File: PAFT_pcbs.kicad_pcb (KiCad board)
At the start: 4 copper layers, 65 x 56.5 mm, 41 parts, among them J1 Servo_R, J10 LinearPotR, J2 Servo_L, J3 Conn_02x03_Top_Bottom, J4 Actuator_L, J5 Actuator_R, J6 RPi_GPIO, J7 LinearPotL, J8 12V_In, J9 RPi_Terminal, SW1 SW_Push, U1 LM2596T-ADJ/LF02, U3 ATtiny85-20P, U4 DRV8848PWP

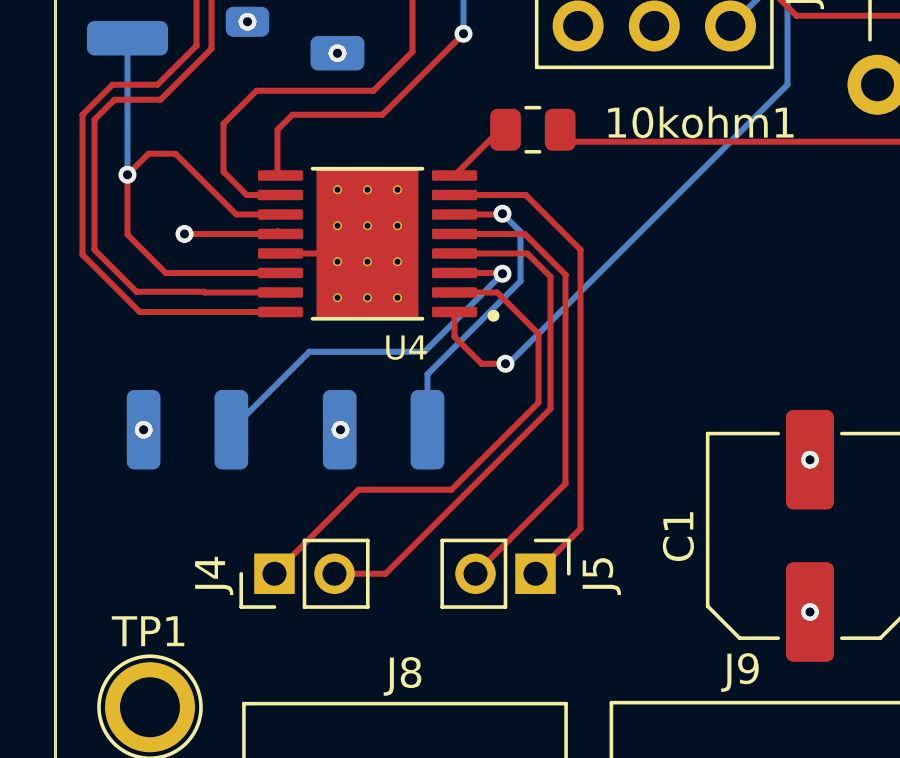
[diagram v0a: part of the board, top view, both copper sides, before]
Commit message: Final updates
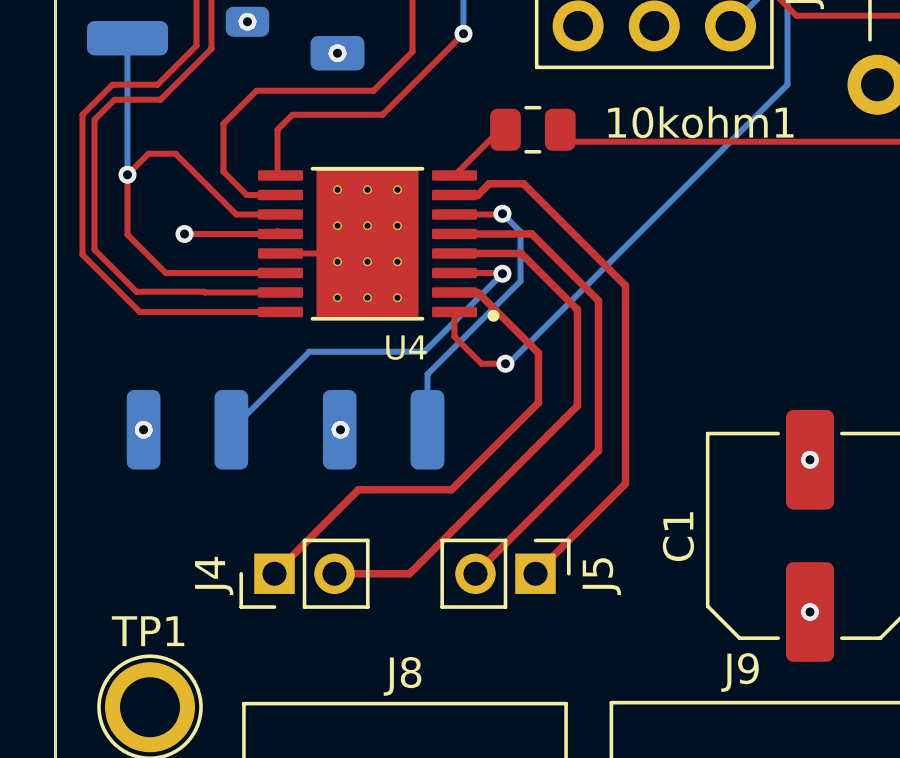
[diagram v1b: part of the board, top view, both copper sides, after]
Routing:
- net /HBridge/BOUT1: track 16.4 -> 18.1 mm
- net /HBridge/AOUT2: track 17.4 -> 18.5 mm
- net /HBridge/BOUT2: track 15.5 -> 16.5 mm
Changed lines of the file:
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@@
 		)
 		(pad_to_mask_clearance 0)
-		(solder_mask_min_width 0.0762)
 		(allow_soldermask_bridges_in_footprints no)
 		(tenting front back)
@@
 			(outputformat 1)
 			(mirror no)
-			(drillshape 1)
+			(drillshape 0)
 			(scaleselection 1)
-			(outputdirectory "")
+			(outputdirectory "../Downloads/")
 		)
 	)
@@
 	)
 	(segment
-		(start 82.3 105)
-		(end 85.2 102.1)
-		(width 0.2)
+		(start 79.2 105)
+		(end 82.3 105)
+		(width 0.25)
 		(layer "F.Cu")
 		(net 18)
 	)
 	(segment
-		(start 85.2 99.8)
-		(end 83.825 98.425)
-		(width 0.2)
+		(start 76.4 107.8)
+		(end 79.2 105)
+		(width 0.25)
 		(layer "F.Cu")
 		(net 18)
 	)
 	(segment
-		(start 83.825 98.425)
-		(end 82.4 98.425)
-		(width 0.2)
+		(start 82.3 105)
+		(end 85.2 102.1)
+		(width 0.25)
 		(layer "F.Cu")
 		(net 18)
 	)
 	(segment
-		(start 85.2 102.1)
-		(end 85.2 99.8)
-		(width 0.2)
+		(start 83.182328 98.425)
+		(end 82.4 98.425)
+		(width 0.25)
 		(layer "F.Cu")
 		(net 18)
 	)
 	(segment
-		(start 79.2 105)
-		(end 82.3 105)
-		(width 0.2)
+		(start 85.2 100.442672)
+		(end 83.182328 98.425)
+		(width 0.25)
 		(layer "F.Cu")
 		(net 18)
 	)
 	(segment
-		(start 76.4 107.8)
-		(end 79.2 105)
-		(width 0.2)
+		(start 85.2 102.1)
+		(end 85.2 100.442672)
+		(width 0.25)
 		(layer "F.Cu")
 		(net 18)
 	)
 	(segment
-		(start 84.825 97.125)
-		(end 85.6 97.9)
-		(width 0.2)
+		(start 86.5 99)
+		(end 86.5 102.2)
+		(width 0.25)
 		(layer "F.Cu")
 		(net 19)
 	)
 	(segment
-		(start 80.1 107.8)
+		(start 80.9 107.8)
 		(end 78.4 107.8)
-		(width 0.2)
+		(width 0.25)
 		(layer "F.Cu")
 		(net 19)
 	)
 	(segment
-		(start 85.6 97.9)
-		(end 85.6 102.3)
-		(width 0.2)
+		(start 86.5 102.2)
+		(end 80.9 107.8)
+		(width 0.25)
 		(layer "F.Cu")
 		(net 19)
 	)
 	(segment
-		(start 85.6 102.3)
-		(end 80.1 107.8)
-		(width 0.2)
+		(start 82.4 97.125)
+		(end 84.625 97.125)
+		(width 0.25)
 		(layer "F.Cu")
 		(net 19)
 	)
 	(segment
-		(start 82.4 97.125)
-		(end 84.825 97.125)
-		(width 0.2)
+		(start 84.625 97.125)
+		(end 86.5 99)
+		(width 0.25)
 		(layer "F.Cu")
 		(net 19)
 	)
 	(segment
-		(start 84.775 95.175)
-		(end 82.4 95.175)
-		(width 0.2)
+		(start 82.4 95.175)
+		(end 83.182328 95.175)
+		(width 0.25)
 		(layer "F.Cu")
 		(net 20)
 	)
 	(segment
-		(start 85.1 107.8)
-		(end 86.6 106.3)
-		(width 0.2)
+		(start 83.557328 94.8)
+		(end 84.7 94.8)
+		(width 0.25)
 		(layer "F.Cu")
 		(net 20)
 	)
 	(segment
-		(start 86.6 97)
-		(end 84.775 95.175)
-		(width 0.2)
+		(start 88.1 98.2)
+		(end 88.1 104.8)
+		(width 0.25)
 		(layer "F.Cu")
 		(net 20)
 	)
 	(segment
-		(start 86.6 106.3)
-		(end 86.6 97)
-		(width 0.2)
+		(start 83.182328 95.175)
+		(end 83.557328 94.8)
+		(width 0.25)
 		(layer "F.Cu")
 		(net 20)
 	)
 	(segment
-		(start 86.101 97.8339)
-		(end 84.7421 96.475)
-		(width 0.2)
+		(start 88.1 104.8)
+		(end 85.1 107.8)
+		(width 0.25)
 		(layer "F.Cu")
-		(net 21)
+		(net 20)
 	)
 	(segment
-		(start 86.1 104.8)
-		(end 86.1 97.8349)
-		(width 0.2)
+		(start 84.7 94.8)
+		(end 88.1 98.2)
+		(width 0.25)
+		(layer "F.Cu")
+		(net 20)
+	)
+	(segment
+		(start 84.975 96.475)
+		(end 82.4 96.475)
+		(width 0.25)
 		(layer "F.Cu")
 		(net 21)
 	)
 	(segment
-		(start 86.1 97.8349)
-		(end 86.101 97.8339)
-		(width 0.2)
+		(start 83.1 107.8)
+		(end 87.2 103.7)
+		(width 0.25)
 		(layer "F.Cu")
 		(net 21)
 	)
 	(segment
-		(start 84.7421 96.475)
-		(end 82.4 96.475)
-		(width 0.2)
+		(start 87.2 98.7)
+		(end 84.975 96.475)
+		(width 0.25)
 		(layer "F.Cu")
 		(net 21)
 	)
 	(segment
-		(start 83.1 107.8)
-		(end 86.1 104.8)
-		(width 0.2)
+		(start 87.2 103.7)
+		(end 87.2 98.7)
+		(width 0.25)
 		(layer "F.Cu")
 		(net 21)
